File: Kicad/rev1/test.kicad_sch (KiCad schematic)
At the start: 74 parts, among them J1 SPKOUT, J2 Tag Con, P1 USB_C_Plug_USB2.0, SW1 SW_Push, SW2 SW_Push, SW4 SW_Push, SW5 SW_Push, U1 MAX98357A, U2 ESP32-S3-WROOM-1, U3 OV5640, U4 24Mhz, U5 AXP2101

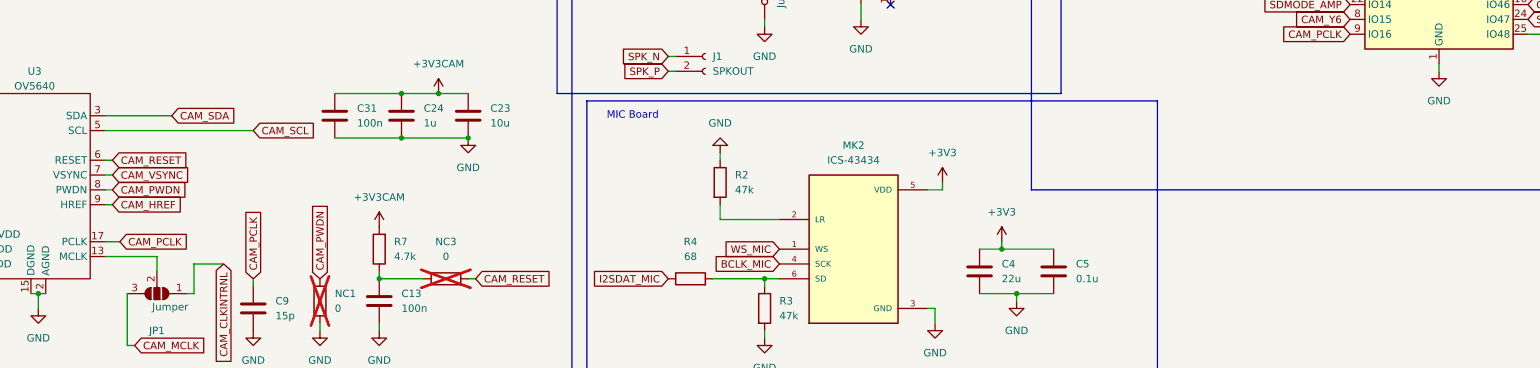
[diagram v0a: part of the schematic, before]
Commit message: Finished REV1 Design and created pcb
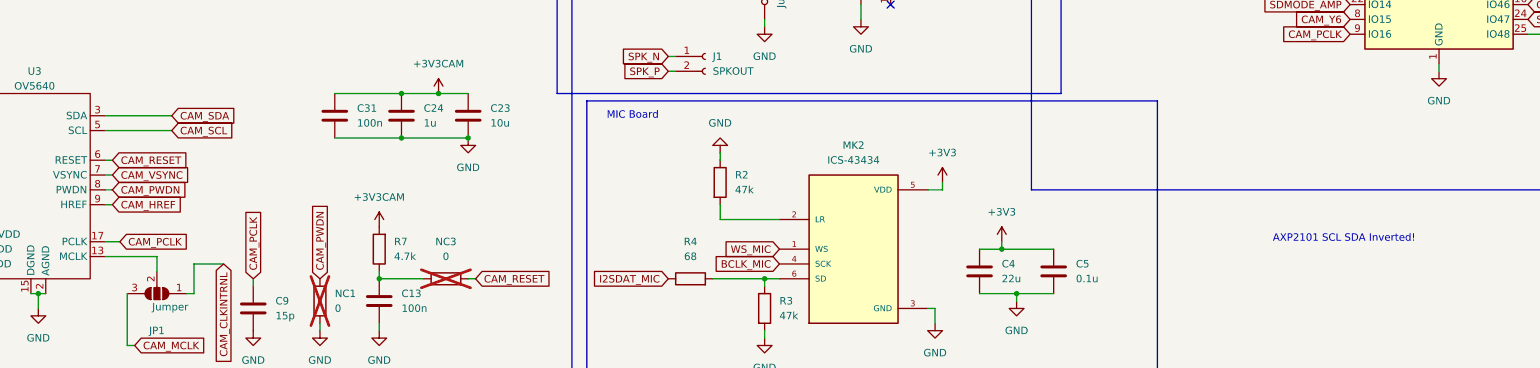
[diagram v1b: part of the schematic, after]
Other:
- note added: "AXP2101 SCL SDA Inverted!"
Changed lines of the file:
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@@
 	(wire
 		(pts
-			(xy 107.95 238.76) (xy 133.35 238.76)
+			(xy 107.95 238.76) (xy 119.38 238.76)
 		)
 		(stroke
@@
 		)
 	)
+	(text "AXP2101 SCL SDA Inverted!"
+		(exclude_from_sim no)
+		(at 320.294 257.302 0)
+		(effects
+			(font
+				(size 1.27 1.27)
+			)
+		)
+	)
 	(text "ESP32 Main Board\n"
 		(exclude_from_sim no)
@@
 	(global_label "CAM_SCL"
 		(shape input)
-		(at 133.35 238.76 0)
-		(fields_autoplaced yes)
-		(effects
-			(font
-				(size 1.27 1.27)
-			)
-			(justify left)
-		)
-		(property "Intersheetrefs" "${INTERSHEET_REFS}"
-			(at 144.6204 238.76 0)
-			(effects
-				(font
+		(at 119.38 238.76 0)
+		(fields_autoplaced yes)
+		(effects
+			(font
+				(size 1.27 1.27)
+			)
+			(justify left)
+		)
+		(property "Intersheetrefs" "${INTERSHEET_REFS}"
+			(at 130.6504 238.76 0)
+			(effects
+				(font
